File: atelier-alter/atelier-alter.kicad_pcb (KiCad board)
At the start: 2 copper layers, 71.4 x 99.5 mm, 28 parts, among them SW1 SW_Push, U1 ATmega32U4-A, Y1 16Mhz

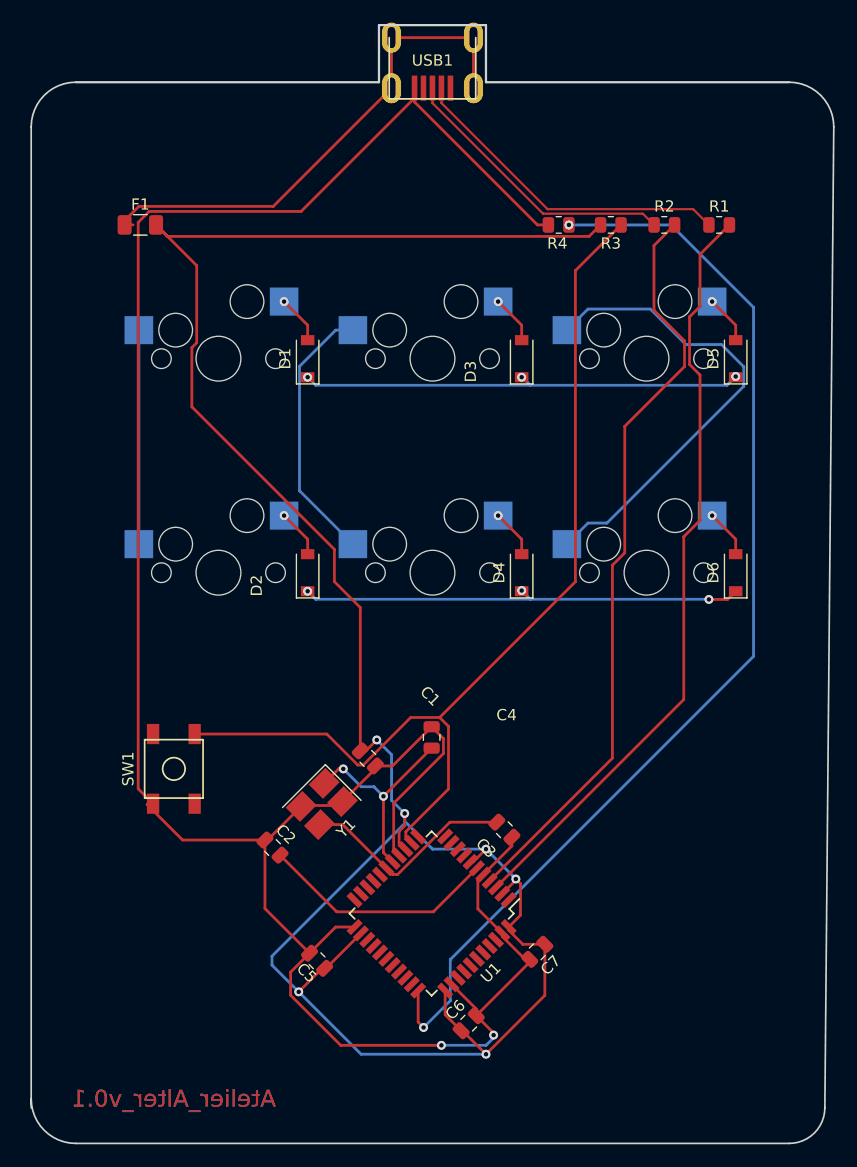
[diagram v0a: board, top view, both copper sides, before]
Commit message: redrawn
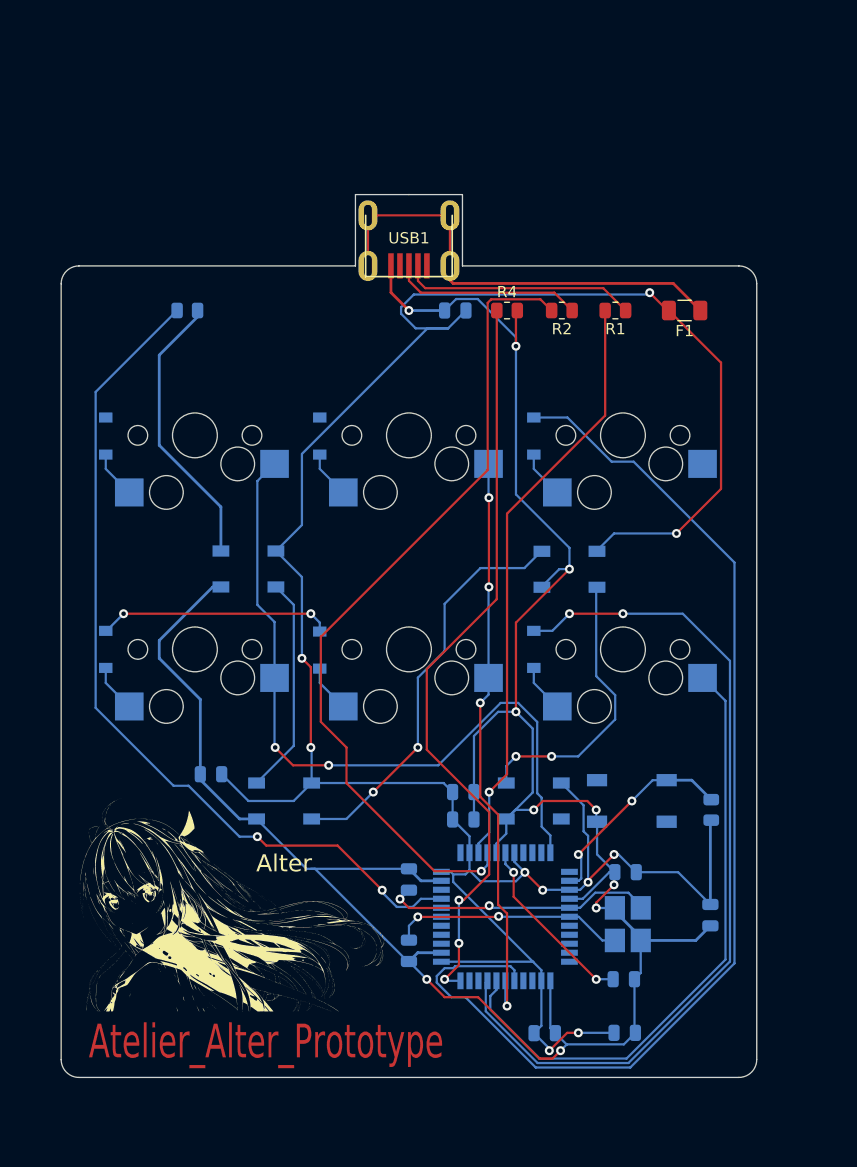
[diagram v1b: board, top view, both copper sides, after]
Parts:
- added Alter: LOGO, Alter_Drawing, F.Cu at (126.2, 120.7)
- added C10: 100nF, Capacitor_SMD:C_0805_2012Metric, B.Cu at (161.3, 132.6)
- added C11: 100nF, Capacitor_SMD:C_0805_2012Metric, B.Cu at (168.9, 122.1)
- added C8: 100nF, Capacitor_SMD:C_0805_2012Metric, B.Cu at (124.5, 109.5)
- added C9: 100nF, Capacitor_SMD:C_0805_2012Metric, B.Cu at (146.2, 68.3)
- added D10: SK6812, LED_SMD:LED_SK6812_PLCC4_5.0x5.0mm_P3.2mm, B.Cu at (153.2, 111.9)
- added D7: SK6812, LED_SMD:LED_SK6812_PLCC4_5.0x5.0mm_P3.2mm, B.Cu at (127.8, 91.3)
- added D8: SK6812, LED_SMD:LED_SK6812_PLCC4_5.0x5.0mm_P3.2mm, B.Cu at (131.0, 111.9)
- added D9: SK6812, LED_SMD:LED_SK6812_PLCC4_5.0x5.0mm_P3.2mm, B.Cu at (156.4, 91.3)
- added R5: 300, Resistor_SMD:R_0805_2012Metric, B.Cu at (122.4, 68.3)
- C1, C3, C4, C5, C6, D1, D2, D3, D4, D5, D6, R3, U1, Y1: moved to B.Cu
- C2: value C_Small -> 1uF; moved to B.Cu
- C7: value 0.1uF -> 10uF; moved to B.Cu
- R1, R2: value R_Small -> 22
- SW1: value SW_Push -> RESET; moved to B.Cu
- moved R3 52.8 mm to (169.0, 112.7), turned to -90 degrees
- moved F1 49.0 mm to (166.6, 68.3), turned to 180 degrees
- moved SW1 40.9 mm to (161.9, 111.9), turned to 180 degrees
- moved C2 33.4 mm to (161.2, 127.8), turned to 180 degrees
- moved Y1 29.3 mm to (161.6, 122.9), turned to -90 degrees
- moved C1 25.1 mm to (161.4, 118.3), turned to 180 degrees
- moved C5 19.9 mm to (146.9, 111.1), turned to 0 degrees
- moved D5 19.2 mm to (153.2, 79.4), turned to -90 degrees
- moved D1 19.2 mm to (115.1, 79.4), turned to -90 degrees
- moved D3 19.2 mm to (134.1, 79.4), turned to -90 degrees
- moved D4 19.2 mm to (134.1, 98.5), turned to -90 degrees
- moved D6 19.2 mm to (153.2, 98.4), turned to -90 degrees
- moved D2 19.2 mm to (115.1, 98.4), turned to -90 degrees
- moved C6 18.1 mm to (146.9, 113.6), turned to 0 degrees
- moved USB1 16.0 mm to (142.1, 59.8)
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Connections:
- U1 pad 11: unconnected-(U1-Pad11) -> COL1
- U1 pad 27: unconnected-(U1-Pad27) -> ROW1
- U1 pad 28: unconnected-(U1-Pad28) -> COL2
- U1 pad 29: unconnected-(U1-Pad29) -> COL3
- U1 pad 30: unconnected-(U1-Pad30) -> ROW2
- U1 pad 41: unconnected-(U1-Pad41) -> UGLOW1
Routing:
- net UGLOW1: track 0.00 -> 76.9 mm, vias 0 -> 2
- net Net-(R3-Pad1): track 88.5 -> 18.7 mm, vias 0 -> 2
- net ROW1: track 40.0 -> 101.3 mm, vias 3 -> 0
- net ROW2: track 39.8 -> 97.6 mm, vias 3 -> 4
- net COL1: track 19.1 -> 65.6 mm, vias 0 -> 2
- net Net-(D8-Pad4): track 0.00 -> 36.4 mm, vias 0 -> 2
- net Net-(R4-Pad1): track 99.2 -> 67.8 mm, vias 2 -> 3
- net COL2: track 23.9 -> 51.9 mm, vias 0 -> 4
- net Net-(D10-Pad2): track 0.00 -> 25.4 mm, vias 0 -> 2
- net Net-(D7-Pad2): track 0.00 -> 25.1 mm
- net +5V: track 201.1 -> 225.8 mm, vias 6 -> 10
- net Net-(D7-Pad4): track 0.00 -> 19.5 mm
- net Net-(R1-Pad2): track 68.3 -> 52.9 mm, vias 0 -> 1
- net COL3: track 41.9 -> 55.1 mm
- net D-: track 29.6 -> 20.9 mm
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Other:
- board size 71.4 x 99.5 mm -> 61.9 x 78.6 mm
- board text added: "Atelier_Alter_Prototype"
- board text removed: "Atelier_Alter_v0.1"
